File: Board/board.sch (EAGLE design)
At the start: 4 parts, among them IC1 L293D

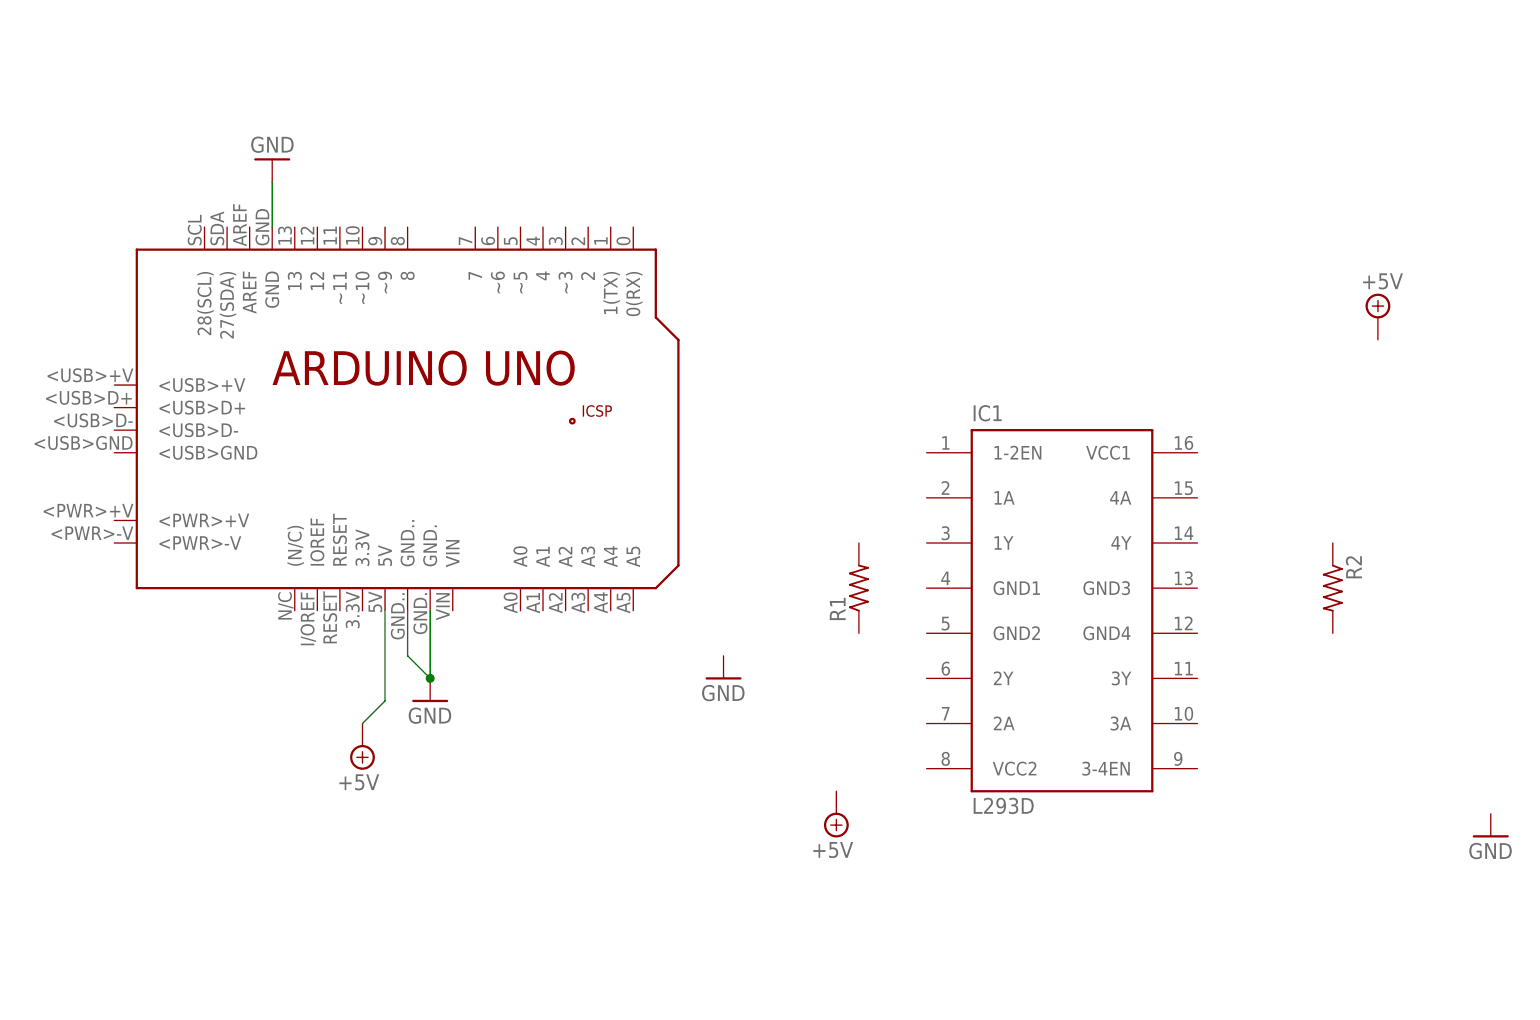
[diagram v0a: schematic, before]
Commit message: various stuff and board
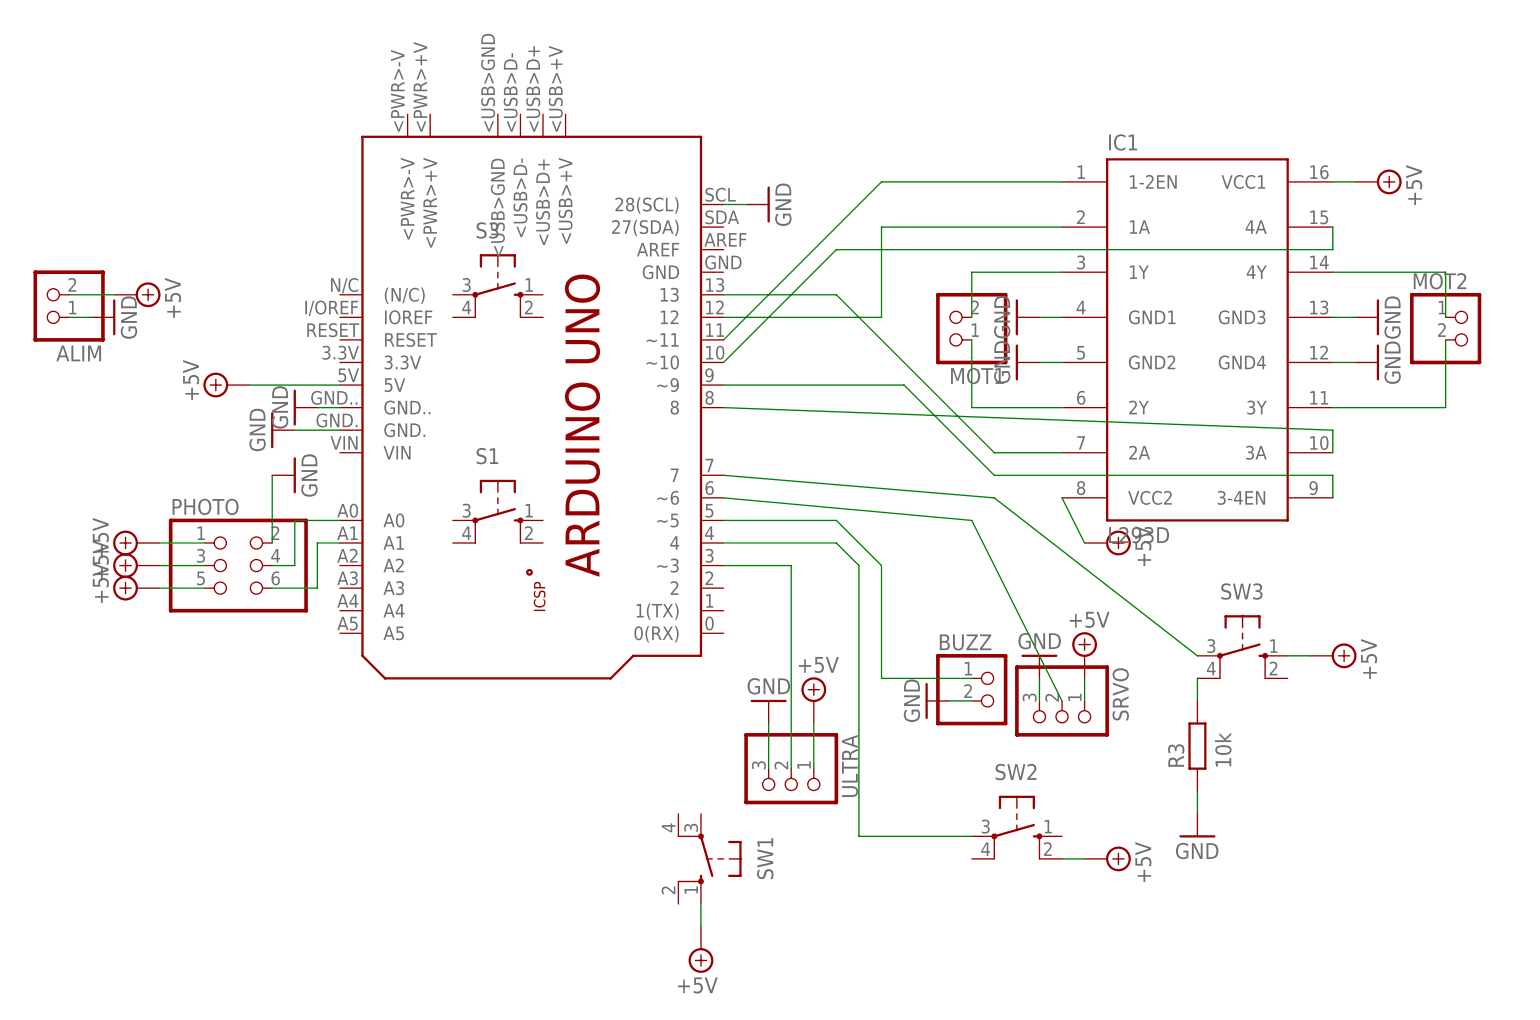
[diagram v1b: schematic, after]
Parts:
- removed R1, R2: (no value), adafruit:R-US_0204/5
- added ALIM, BUZZ, MOT1, MOT2: (no value), pinhead:PINHD-1X2
- added PHOTO: (no value), pinhead:PINHD-2X3
- added R3: 10k, BaseApp:RESISTOR
- added S1, S3, SW1, SW2, SW3: (no value), adafruit:40-XX
- added SRVO, ULTRA: (no value), pinhead:PINHD-1X3
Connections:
- new net N$1: IC1.1Y, MOT1.2
- new net N$10: IC1.1-2EN, PCB1.~11
- new net N$11: PCB1.A1, PHOTO.6
- new net N$12: PCB1.A0, PHOTO.4
- new net N$13: PHOTO.2
- new net N$14: PCB1.~6, SRVO.2
- new net N$15: PCB1.~3, ULTRA.2
- new net N$16: BUZZ.1, PCB1.~5
- new net N$17: PCB1.7, SW3.P
- new net N$18: R3.2, SW3.P1
- new net N$19: PCB1.4, SW2.P
- new net N$2: IC1.2Y, MOT1.1
- new net N$3: IC1.3Y, MOT2.2
- new net N$4: IC1.4Y, MOT2.1
- new net N$5: IC1.1A, PCB1.12
- new net N$6: IC1.2A, PCB1.13
- new net N$7: IC1.4A, PCB1.~10
- new net N$8: IC1.3-4EN, PCB1.~9
- new net N$9: IC1.3A, PCB1.8
- net +5V: now also ALIM.2, IC1.VCC1, IC1.VCC2, PHOTO.1, PHOTO.3, PHOTO.5, SRVO.1, SW1.S, SW2.S1, SW3.S, ULTRA.1
- net GND: now also ALIM.1, BUZZ.2, IC1.GND1, IC1.GND2, IC1.GND3, IC1.GND4, PCB1.28(SCL), R3.1, SRVO.3, ULTRA.3; no longer PCB1.GND
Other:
- moved on the sheet: IC1
